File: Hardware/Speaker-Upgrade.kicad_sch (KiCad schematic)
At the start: 34 parts, among them J1 POWER, J2 CONN_PCB1, J3 CONN_PCB2, J4 AUDIO_JACK, SW1 SW_Slide, U1 LM7805, U2 WIN-668, U3 AN7522N

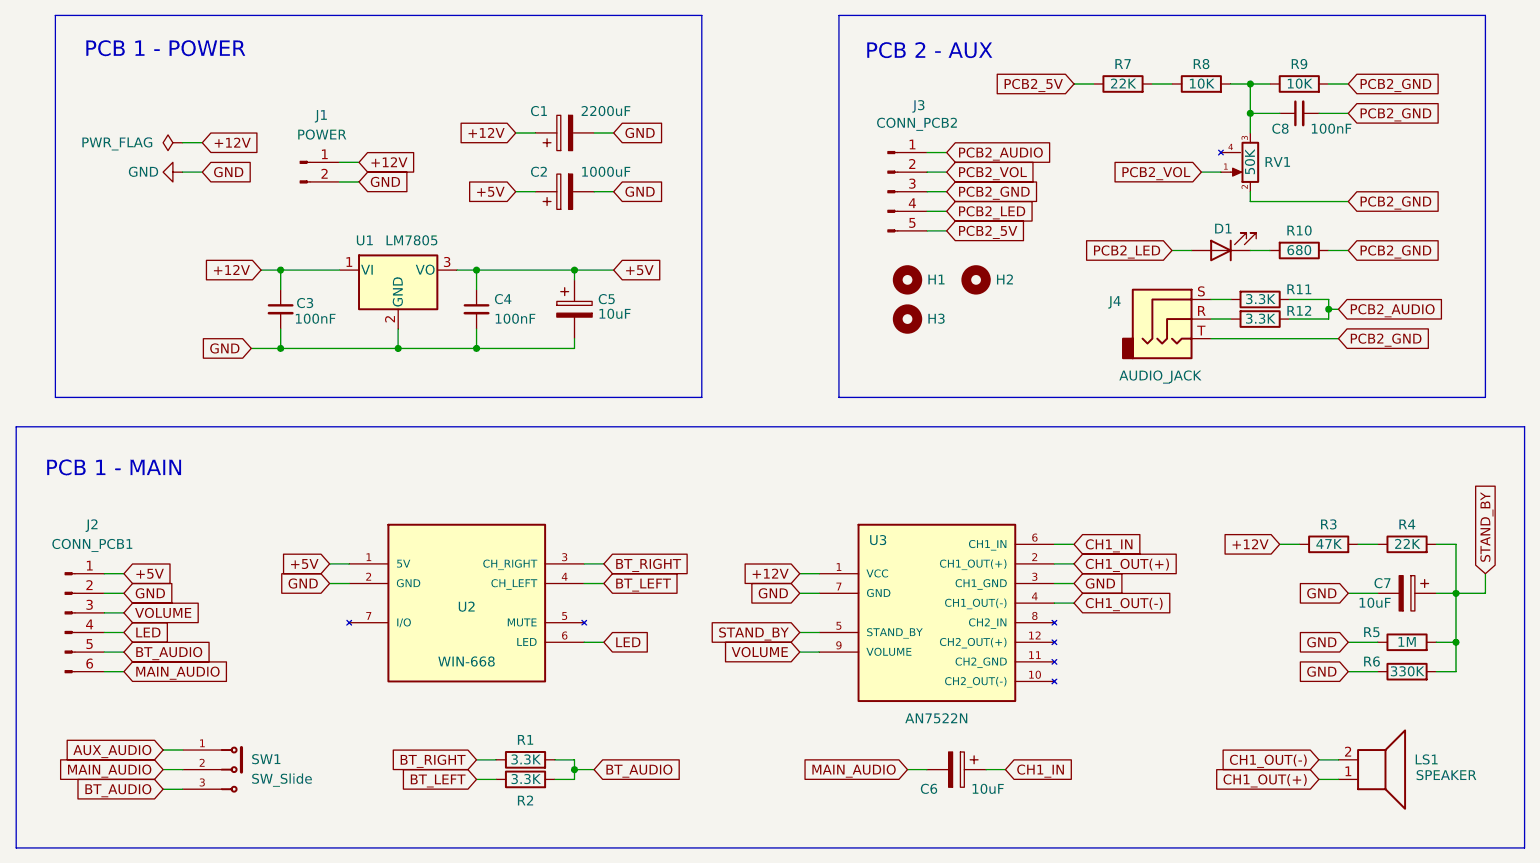
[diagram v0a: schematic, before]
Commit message: Improvements on schematics and PCB
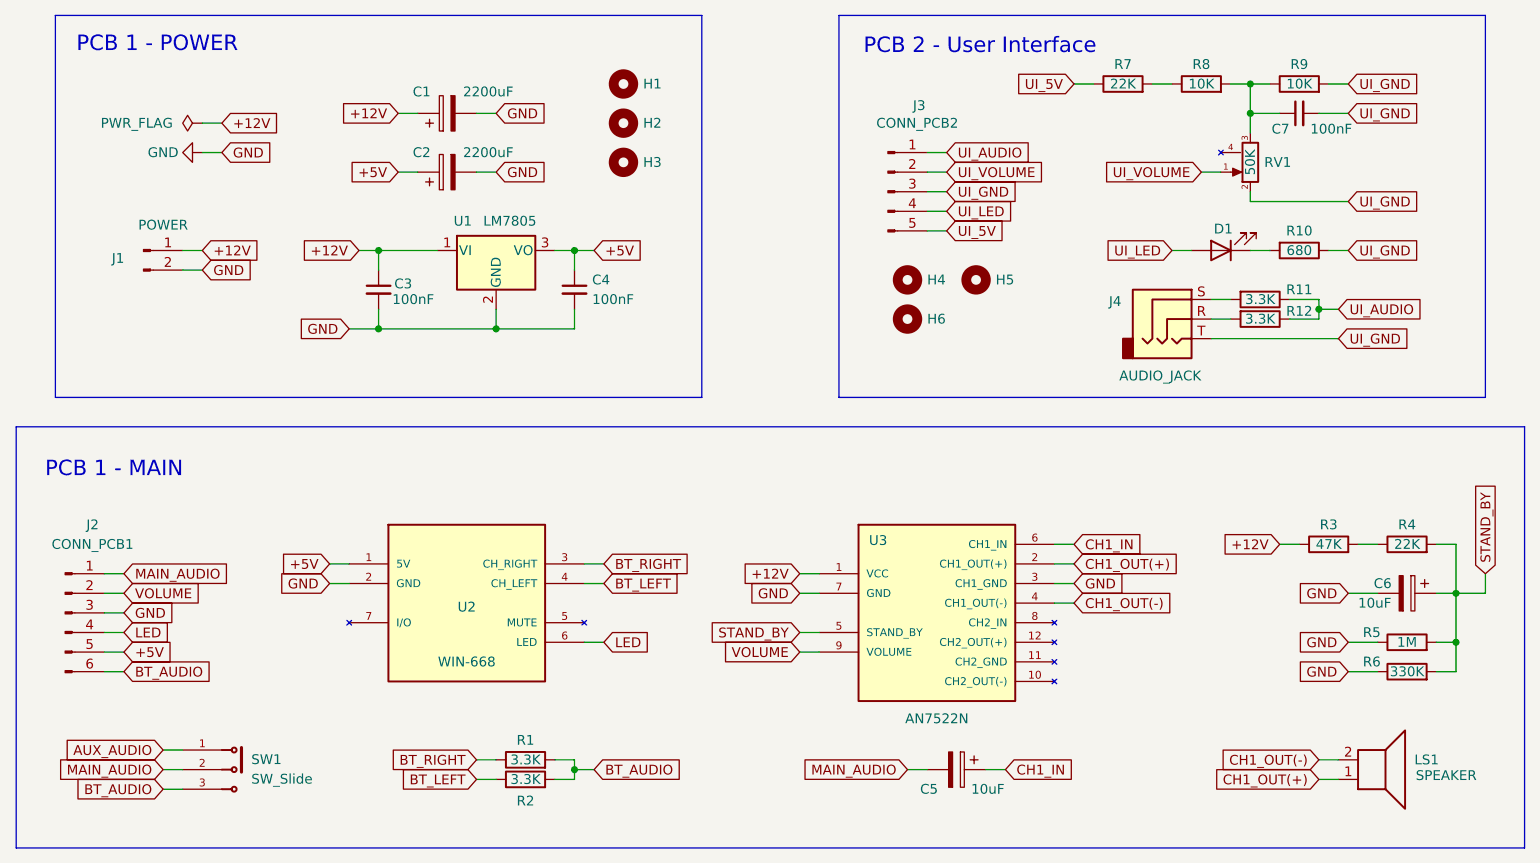
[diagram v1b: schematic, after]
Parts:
- removed C5: 10uF, Capacitor_THT:C_Radial_D10.0mm_H16.0mm_P5.00mm, symbol Device:C_Polarized
- added H1, H2, H3: MountingHole, MountingHole:MountingHole_2.2mm_M2, symbol Mechanical:MountingHole
- C2: value 1000uF -> 2200uF; footprint Capacitor_THT:C_Radial_D10.0mm_H12.5mm_P5.00mm -> Capacitor_THT:C_Radial_D10.0mm_H16.0mm_P5.00mm
- C5: renamed from C6; footprint Capacitor_THT:C_Radial_D6.3mm_H11.0mm_P2.50mm -> Capacitor_THT:C_Radial_D10.0mm_H16.0mm_P5.00mm
- J2: footprint Connector_JST:JST_EH_B6B-EH-A_1x06_P2.50mm_Vertical -> Connector_PinHeader_2.54mm:PinHeader_2x06_P2.54mm_Vertical
- R5, R6: footprint Resistor_THT:R_Axial_DIN0207_L6.3mm_D2.5mm_P2.54mm_Vertical -> Resistor_THT:R_Axial_DIN0207_L6.3mm_D2.5mm_P7.62mm_Horizontal
- renumbered C7 to C6, C8 to C7, H1 to H4, H2 to H5, H3 to H6
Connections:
- net +5V: now also J2.5 (Pin_5); no longer J2.1 (Pin_1)
- net BT_AUDIO: now also J2.6 (Pin_6); no longer J2.5 (Pin_5)
- net GND: now also J2.3 (Pin_3); no longer J2.2 (Pin_2)
- net MAIN_AUDIO: now also J2.1 (Pin_1); no longer J2.6 (Pin_6)
- net VOLUME: now also J2.2 (Pin_2); no longer J2.3 (Pin_3)
- net PCB2_5V renamed UI_5V
- net PCB2_AUDIO renamed UI_AUDIO
- net PCB2_GND renamed UI_GND
- net PCB2_LED renamed UI_LED
- net PCB2_VOL renamed UI_VOLUME
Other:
- note added: "PCB 2 - User Interface"
- note removed: "PCB 2 - AUX"
- moved on the sheet: C1, C2, C3, C4, J1, U1

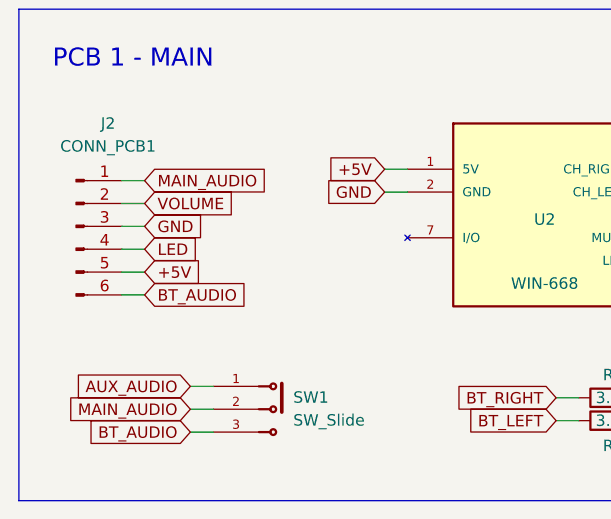
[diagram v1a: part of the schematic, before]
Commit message: Improvements on schematics and PCB
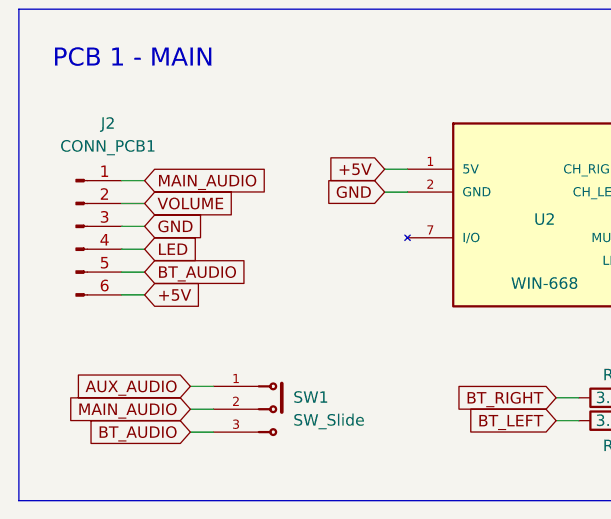
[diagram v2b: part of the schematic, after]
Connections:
- net +5V: now also J2.6 (Pin_6); no longer J2.5 (Pin_5)
- net BT_AUDIO: now also J2.5 (Pin_5); no longer J2.6 (Pin_6)

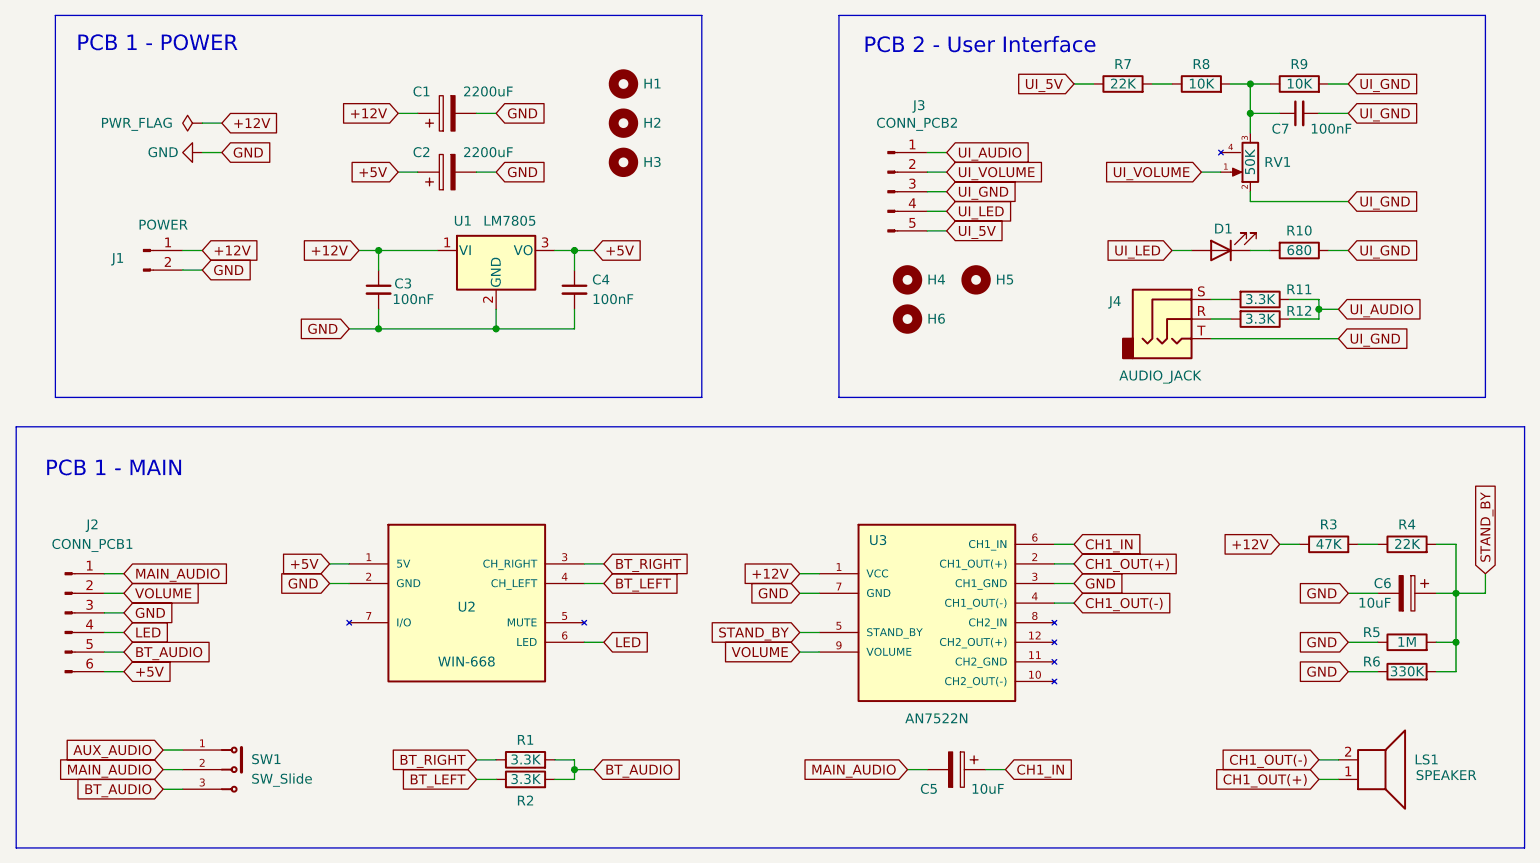
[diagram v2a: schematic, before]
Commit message: Minor improvements on schematics and PCB
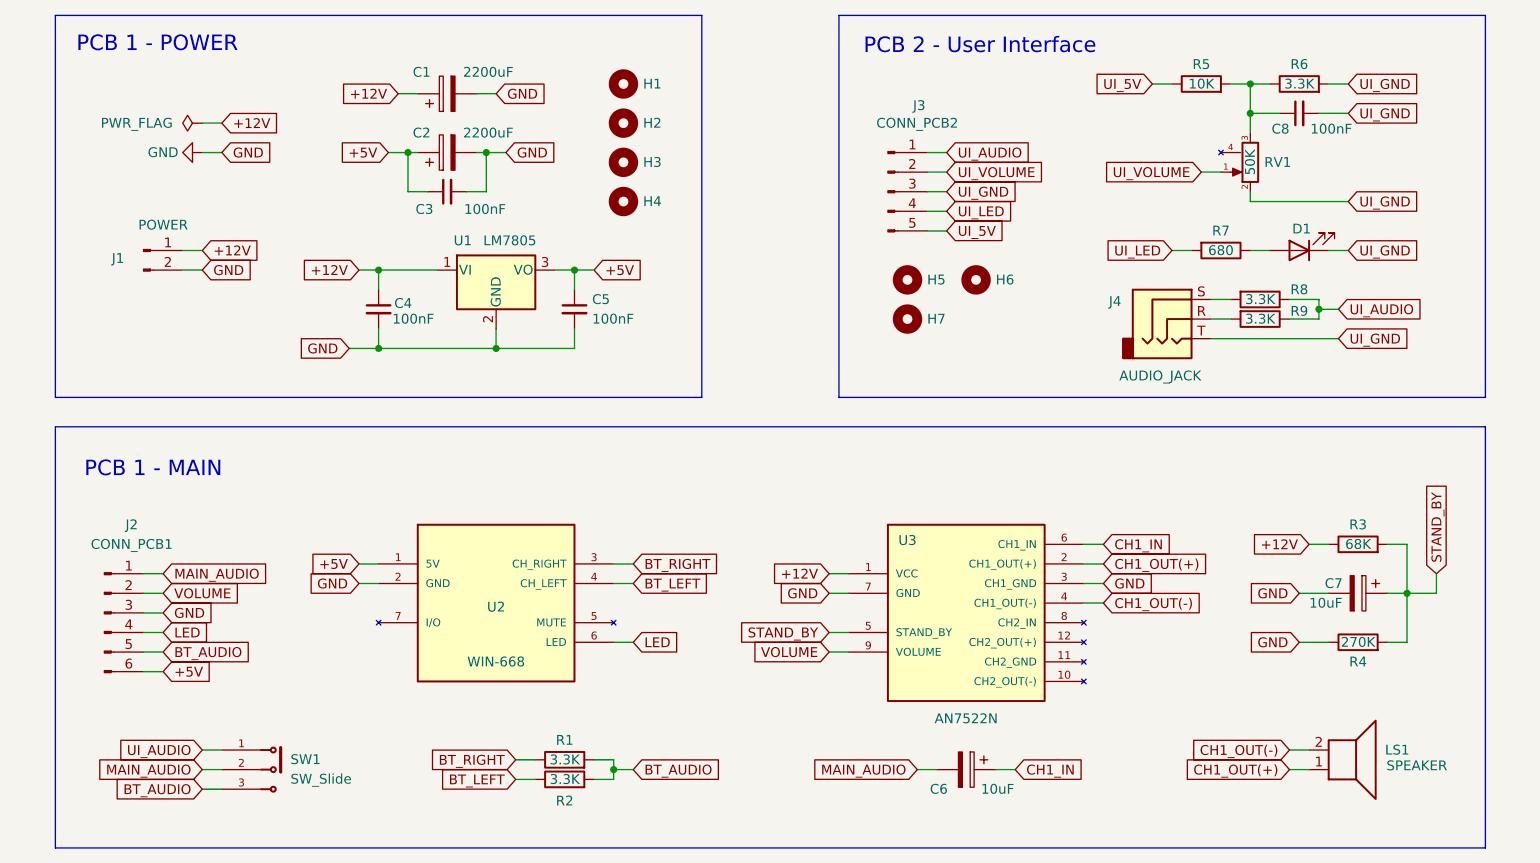
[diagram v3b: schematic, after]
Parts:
- removed R4: 22K, Resistor_THT:R_Axial_DIN0207_L6.3mm_D2.5mm_P2.54mm_Vertical, symbol Device:R
- removed R6: 330K, Resistor_THT:R_Axial_DIN0207_L6.3mm_D2.5mm_P7.62mm_Horizontal, symbol Device:R
- removed R8: 10K, Resistor_THT:R_Axial_DIN0207_L6.3mm_D2.5mm_P7.62mm_Horizontal, symbol Device:R
- added C3: 100nF, Capacitor_THT:C_Disc_D6.0mm_W2.5mm_P5.00mm, symbol Device:C_Small
- added H4: MountingHole, MountingHole:MountingHole_2.2mm_M2, symbol Mechanical:MountingHole
- R3: value 47K -> 68K
- R4: renamed from R5; value 1M -> 270K; footprint Resistor_THT:R_Axial_DIN0207_L6.3mm_D2.5mm_P7.62mm_Horizontal -> Resistor_THT:R_Axial_DIN0207_L6.3mm_D2.5mm_P2.54mm_Vertical
- R5: renamed from R7; value 22K -> 10K
- R6: renamed from R9; value 10K -> 3.3K
- renumbered C3 to C4, C4 to C5, C5 to C6, C6 to C7, C7 to C8, H4 to H5, H5 to H6, H6 to H7, R10 to R7, R11 to R8, R12 to R9
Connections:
- net AUX_AUDIO is gone; now on net UI_AUDIO: SW1.1
- net +5V: now also C3.1
- net GND: now also C3.2
- net STAND_BY: now also R3.2
- net UI_GND: now also D1.1 (K); no longer R7.1
- net UI_LED: now also R7.2; no longer D1.2 (A)
- net at C8.1, R6.1, RV1.3: now also R5.2
- new net: D1.2 (A), R7.1
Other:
- moved on the sheet: C1, C2, C4, C5, C6, C7, D1, J2, LS1, R1, R2, R3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

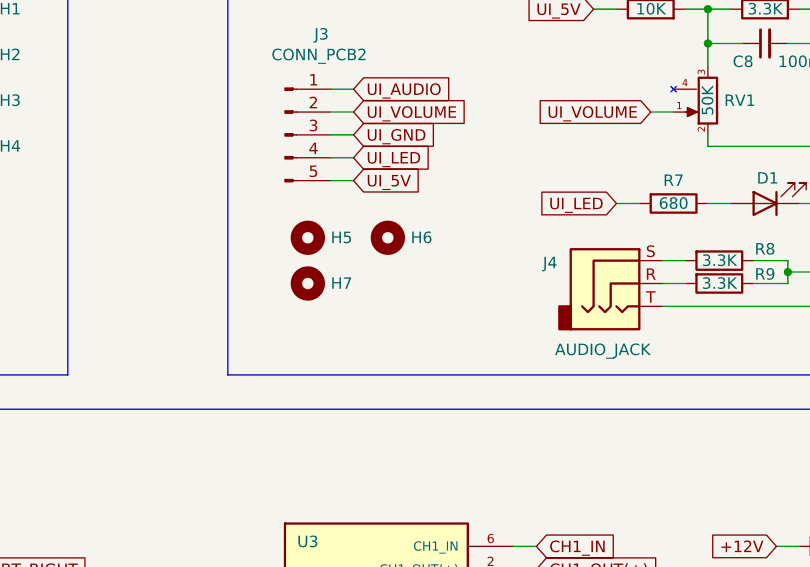
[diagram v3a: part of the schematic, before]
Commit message: Minor improvements on schematics and PCB
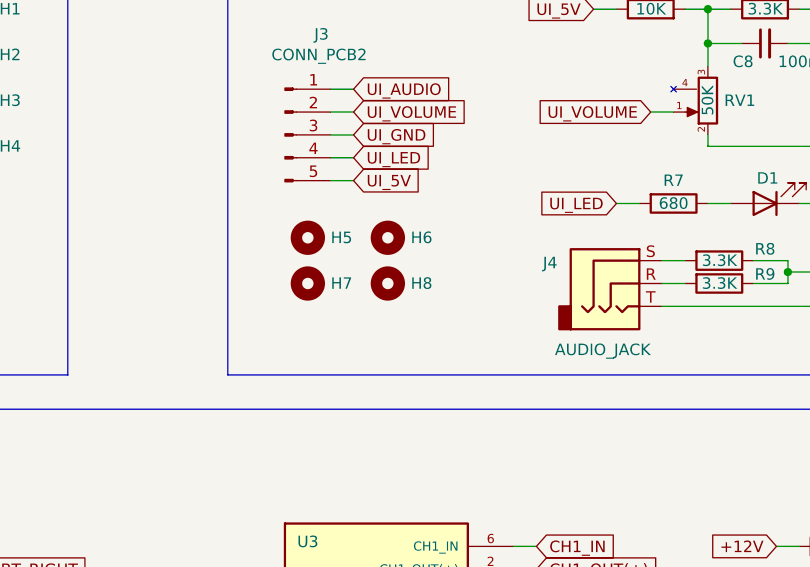
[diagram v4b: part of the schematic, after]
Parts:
- added H8: MountingHole, MountingHole:MountingHole_2.2mm_M2, symbol Mechanical:MountingHole
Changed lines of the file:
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@@
+	)
+	(symbol
+		(lib_id "Mechanical:MountingHole")
+		(at 172.72 72.39 0)
+		(unit 1)
+		(exclude_from_sim no)
+		(in_bom no)
+		(on_board yes)
+		(dnp no)
+		(property "Reference" "H8"
+			(at 175.26 72.39 0)
+			(effects
+				(font
+					(size 1.27 1.27)
+				)
+				(justify left)
+			)
+		)
+		(property "Value" "MountingHole"
+			(at 175.26 73.6599 0)
+			(effects
+				(font
+					(size 1.27 1.27)
+				)
+				(justify left)
+				(hide yes)
+			)
+		)
+		(property "Footprint" "MountingHole:MountingHole_2.2mm_M2"
+			(at 172.72 72.39 0)
+			(effects
+				(font
+					(size 1.27 1.27)
+				)
+				(hide yes)
+			)
+		)
+		(property "Datasheet" "~"
+			(at 172.72 72.39 0)
+			(effects
+				(font
+					(size 1.27 1.27)
+				)
+				(hide yes)
+			)
+		)
+		(property "Description" "Mounting Hole without connection"
+			(at 172.72 72.39 0)
+			(effects
+				(font
+					(size 1.27 1.27)
+				)
+				(hide yes)
+			)
+		)
+		(instances
+			(project "Speaker-Upgrade"
+				(path "/c7d8bf82-cc6e-452e-b6b1-216b46c84a4f"
+					(reference "H8")
+					(unit 1)
+				)
+			)
+		)
 	)
 	(symbol
